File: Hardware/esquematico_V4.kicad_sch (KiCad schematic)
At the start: 19 parts, among them J11 Conn_01x02_Socket, J14 Conn_01x02_Socket, J15 Conn_01x02_Socket, J16 Conn_01x02_Socket, J23 RJ45, J24 RJ45, J25 RJ45, J4 Conn_cartao_SD, J5 Conn_BH1750, J6 Conn_BMP, U2 module_bh1750, U3 module_bme280, U6 MicroSD Card Adapter, U7 NUCLEO-F446RE

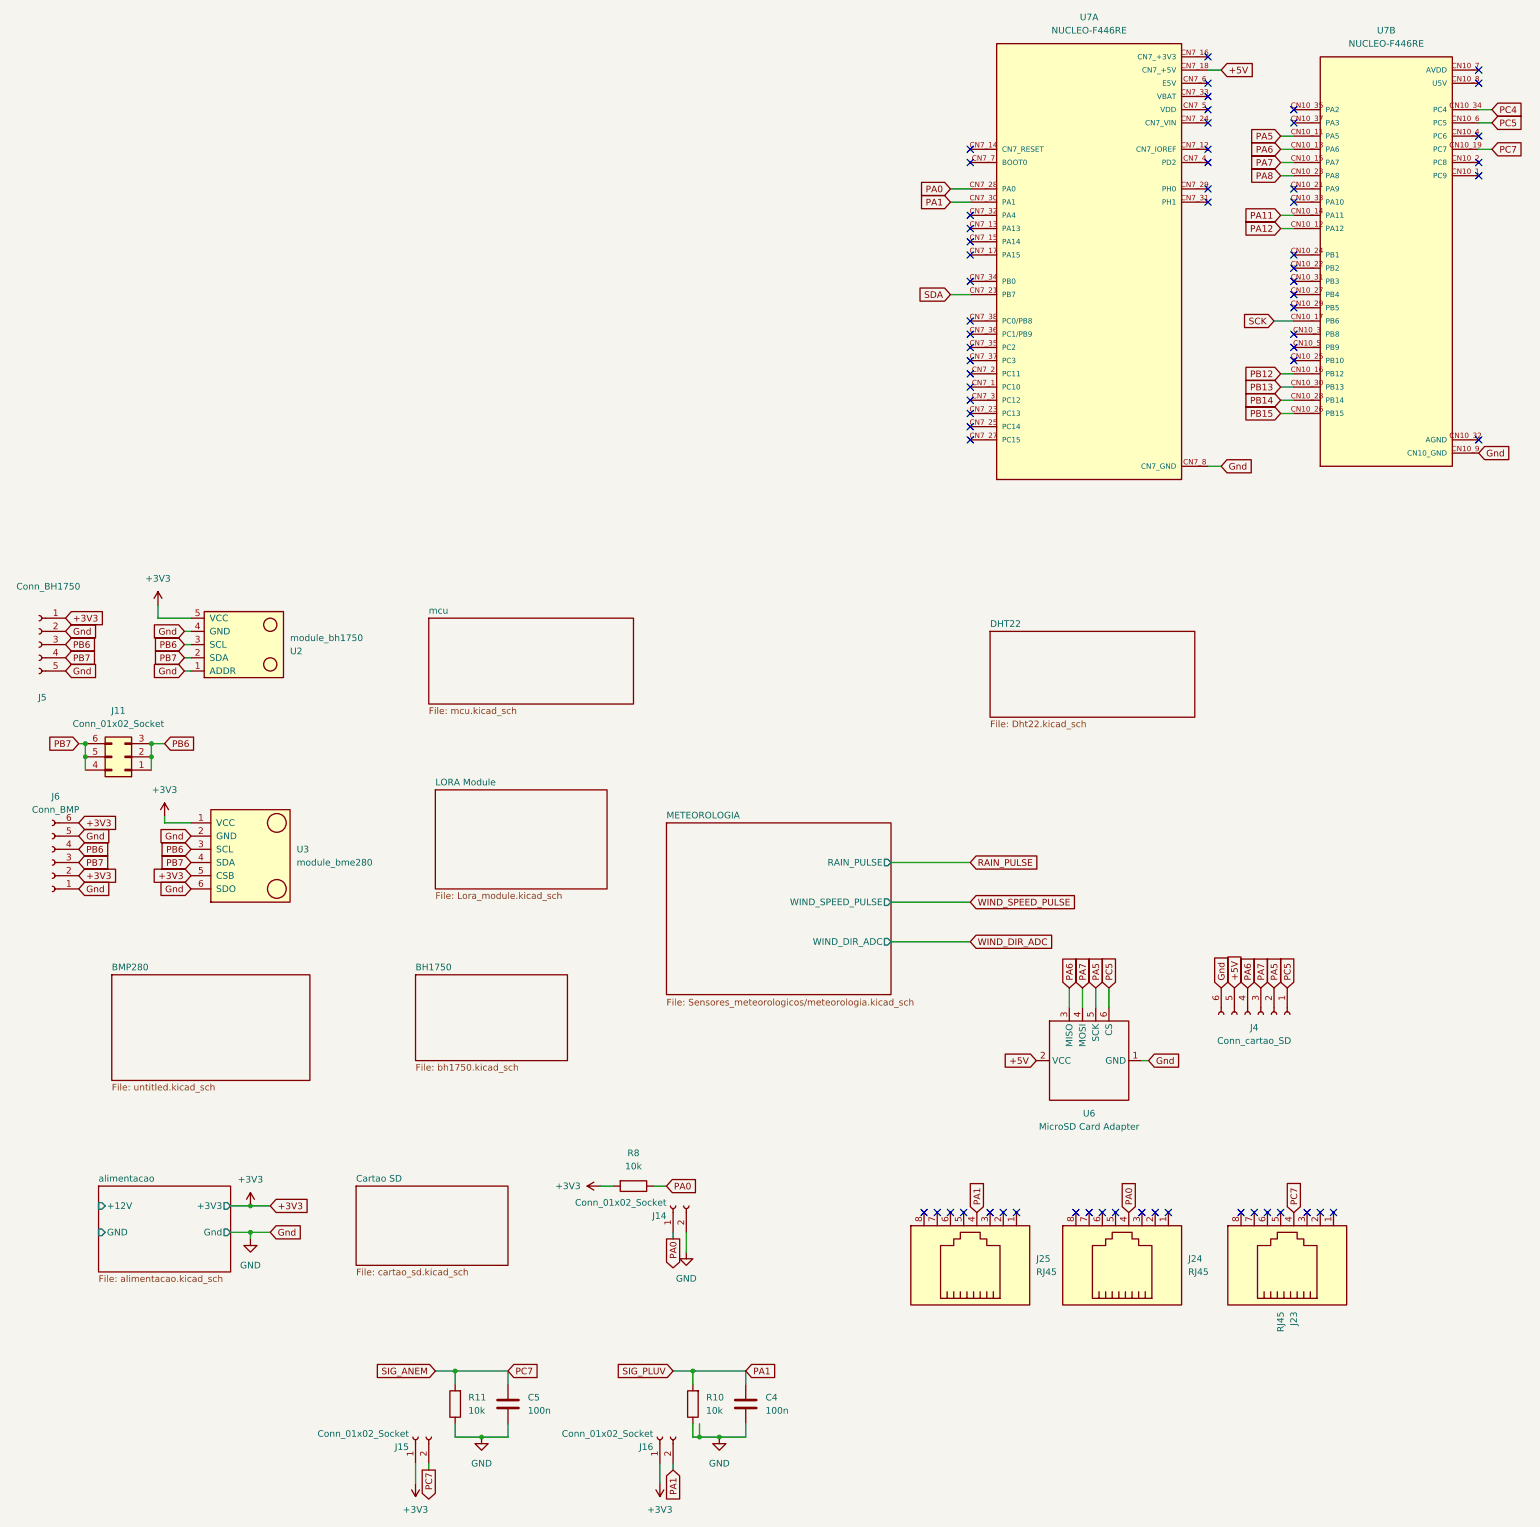
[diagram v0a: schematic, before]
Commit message: Sensores metereologicos -IA que fez
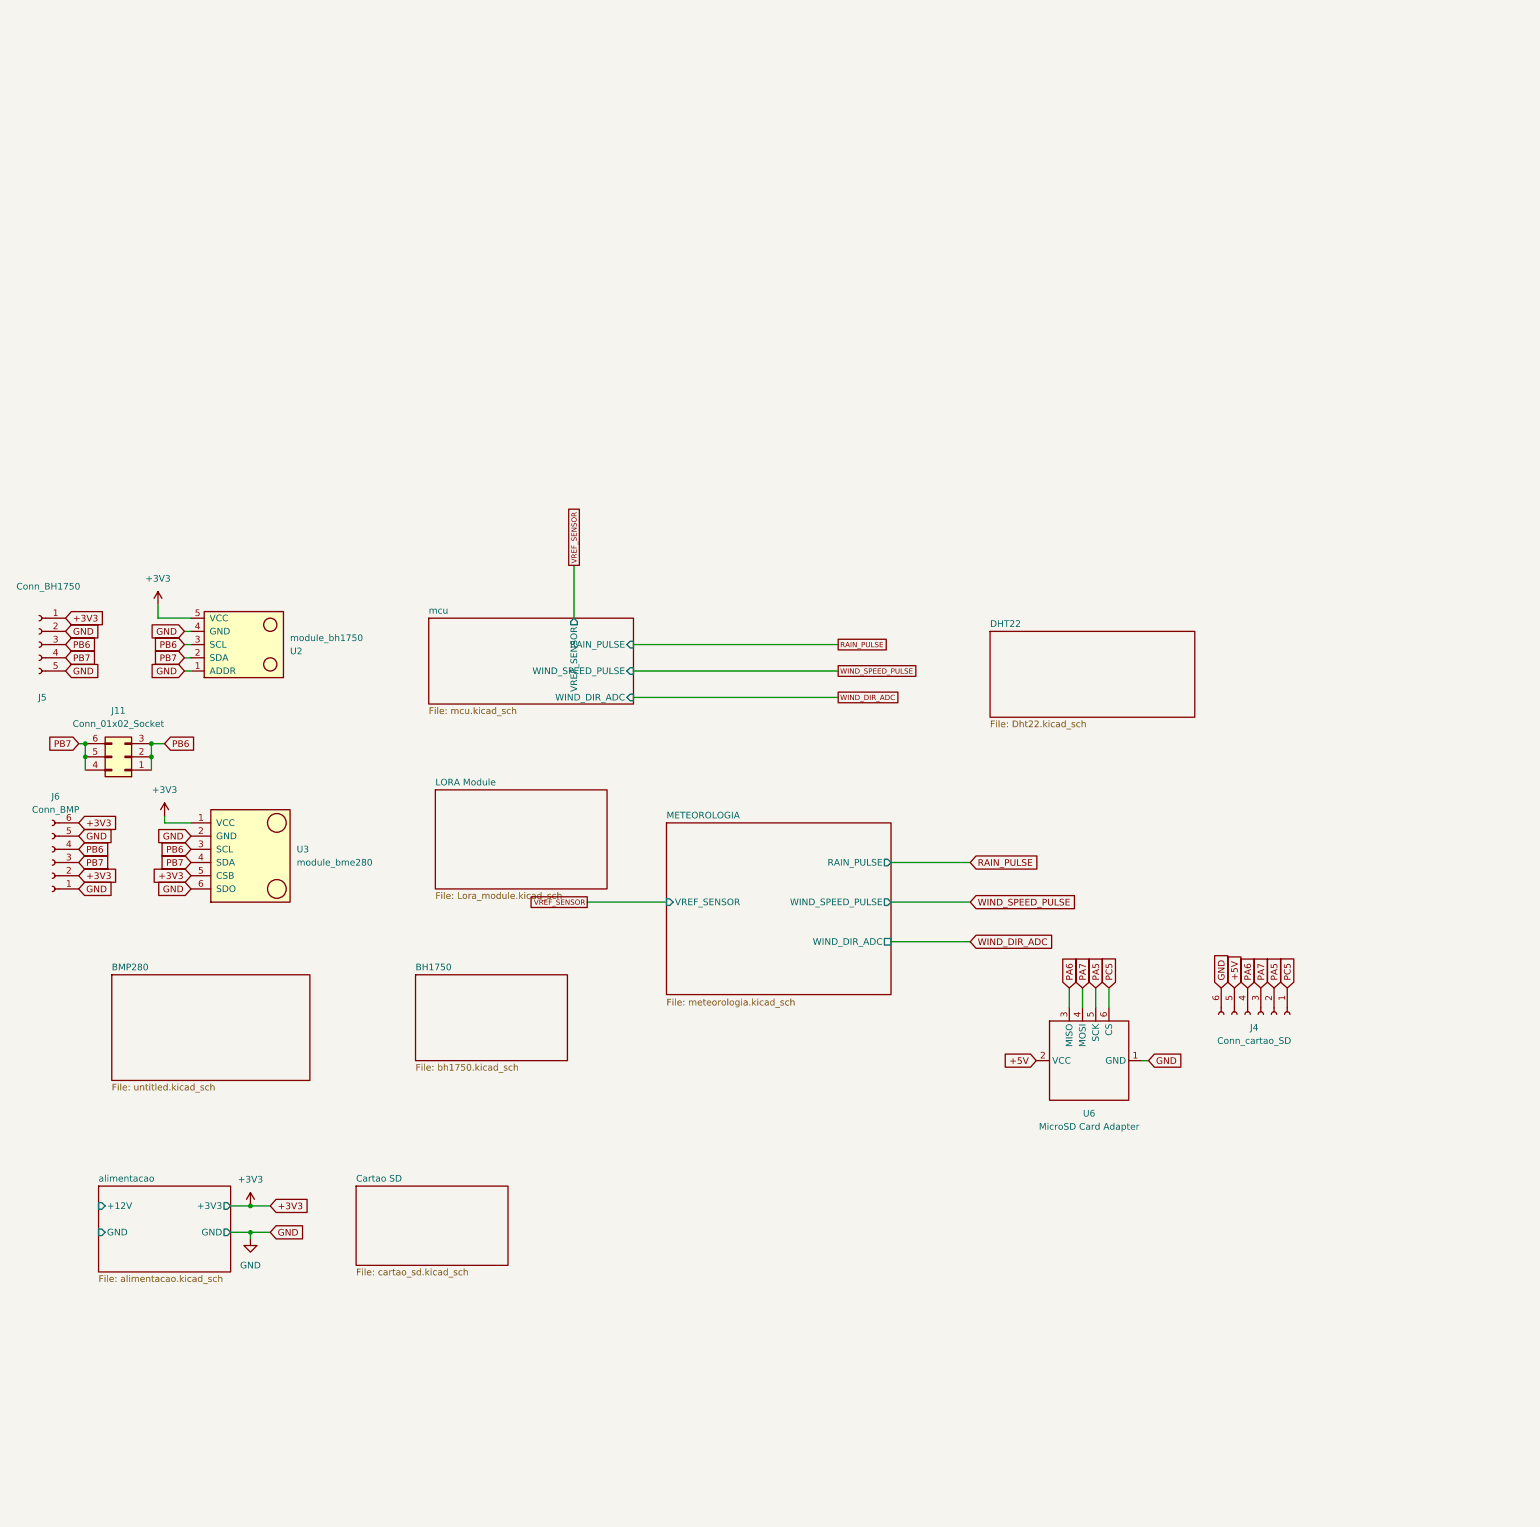
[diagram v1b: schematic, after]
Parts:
- removed C4, C5: 100n, Capacitor_THT:C_Disc_D3.8mm_W2.6mm_P2.50mm, symbol Device:C
- removed J14, J15, J16: Conn_01x02_Socket, Connector_PinSocket_2.54mm:PinSocket_1x02_P2.54mm_Vertical, symbol Connector:Conn_01x02_Socket
- removed J23, J24, J25: RJ45, Connector_RJ:RJ45_RCH_RC01937, symbol Connector:RJ45
- removed R10, R11, R8: 10k, Resistor_THT:R_Axial_DIN0204_L3.6mm_D1.6mm_P7.62mm_Horizontal, symbol Device:R
- removed U7: NUCLEO-F446RE, myLibrary:MODULE_NUCLEO-F446RE, symbol Nucleo_F446:NUCLEO-F446RE
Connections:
- net CN10_GND renamed GND
- no-connect marks 65 -> 0
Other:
- sheet METEOROLOGIA: file Sensores_meteorologicos/meteorologia.kicad_sch -> meteorologia.kicad_sch
- sheet METEOROLOGIA ports: added VREF_SENSOR; removed none
- sheet alimentacao ports: added none; removed Gnd
- sheet mcu ports: added RAIN_PULSE, VREF_SENSOR, WIND_DIR_ADC, WIND_SPEED_PULSE; removed none
